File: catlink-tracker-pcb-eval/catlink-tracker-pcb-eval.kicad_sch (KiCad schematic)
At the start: 41 parts, among them J1 S2B-PH-K, J2 U.FL, J3 Header_01x03, J4 Header_02x02, J5 Header_02x03, J6 Header_01x02, J7 Header_01x06, J8 Header_01x05, SW1 SW_Push, U1 STM32L412K8Tx, U2 TLV75530PDBV, U3 Ai-Thinker-Ra-01S, U4 E108-GN03

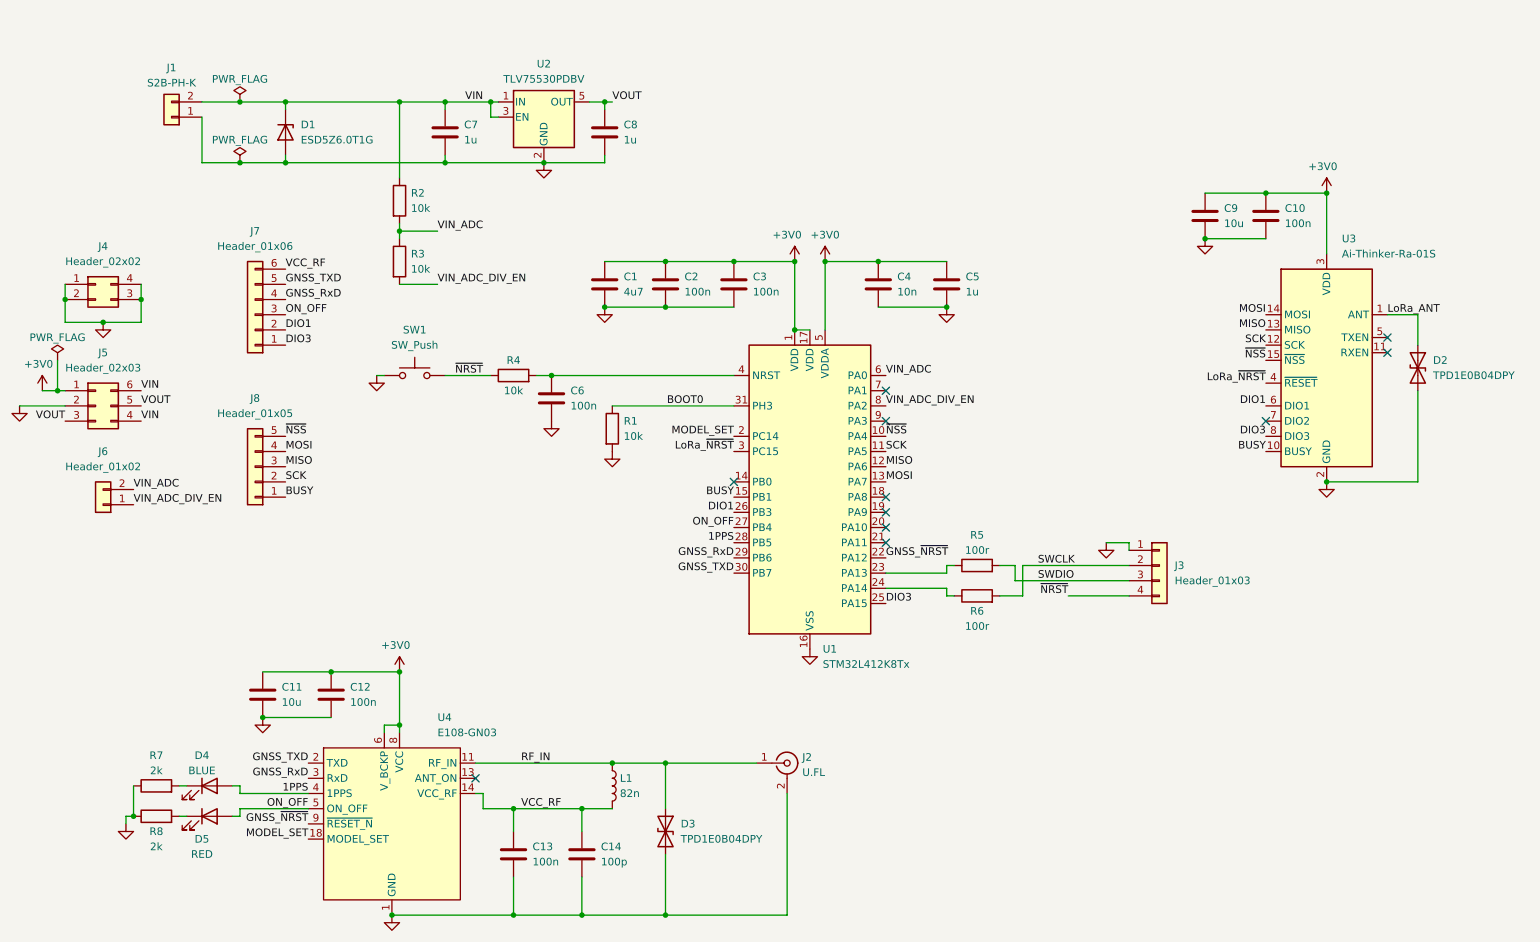
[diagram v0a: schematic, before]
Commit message: v0.1
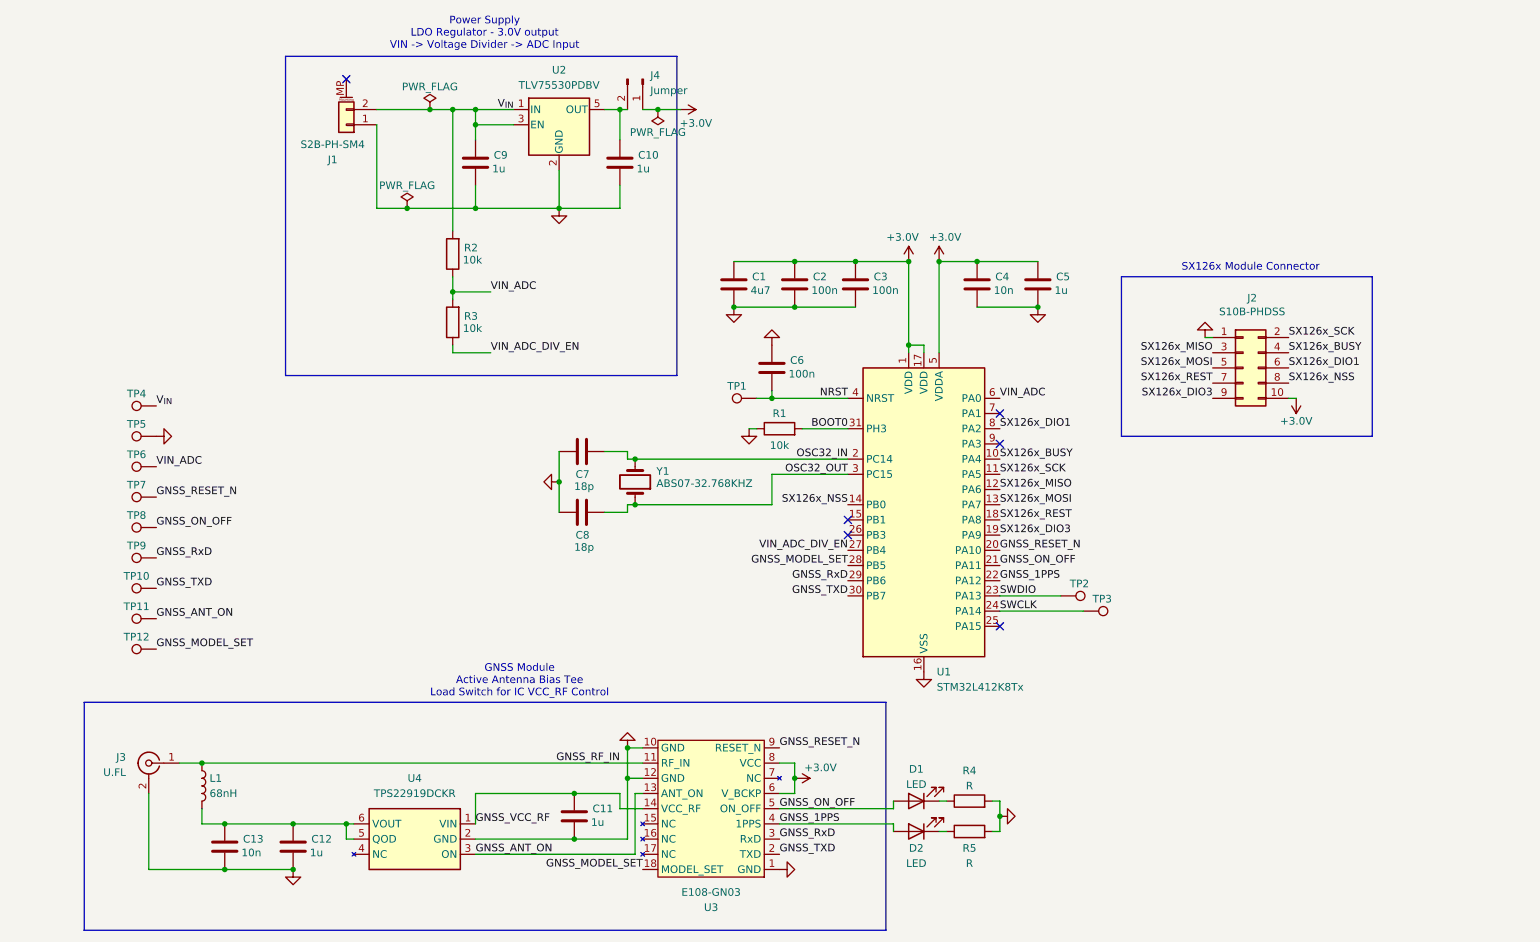
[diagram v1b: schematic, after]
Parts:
- removed C14: 100p, Custom:C_0603_1608Metric, symbol Device:C
- removed D1: ESD5Z6.0T1G, Custom:D_SOD-523, symbol Device:D_Zener
- removed D2, D3: TPD1E0B04DPY, Custom:D_Texas_DPY0002A_0.6x1mm_P0.65mm, symbol Device:D_TVS
- removed D4: BLUE, LED_THT:LED_D3.0mm, symbol Device:LED
- removed D5: RED, LED_THT:LED_D3.0mm, symbol Device:LED
- removed J1: S2B-PH-K, Connector_JST:JST_PH_S2B-PH-K_1x02_P2.00mm_Horizontal, symbol Connector_Generic:Conn_01x02
- removed J2: U.FL, Connector_Coaxial:U.FL_Hirose_U.FL-R-SMT-1_Vertical, symbol Connector:Conn_Coaxial
- removed J3: Header_01x03, Connector_PinHeader_2.54mm:PinHeader_1x04_P2.54mm_Vertical, symbol Connector_Generic:Conn_01x04
- removed J4: Header_02x02, Connector_PinHeader_2.54mm:PinHeader_2x02_P2.54mm_Vertical, symbol Connector_Generic:Conn_02x02_Counter_Clockwise
- removed J5: Header_02x03, Connector_PinHeader_2.54mm:PinHeader_2x03_P2.54mm_Vertical, symbol Connector_Generic:Conn_02x03_Counter_Clockwise
- removed J6: Header_01x02, Connector_PinHeader_2.54mm:PinHeader_1x02_P2.54mm_Vertical, symbol Connector_Generic:Conn_01x02
- removed J7: Header_01x06, Connector_PinHeader_2.54mm:PinHeader_1x06_P2.54mm_Vertical, symbol Connector_Generic:Conn_01x06
- removed J8: Header_01x05, Connector_PinHeader_2.54mm:PinHeader_1x05_P2.54mm_Vertical, symbol Connector_Generic:Conn_01x05
- removed R6: 100r, Custom:R_0603_1608Metric, symbol Device:R
- removed R7, R8: 2k, Resistor_THT:R_Axial_DIN0204_L3.6mm_D1.6mm_P1.90mm_Vertical, symbol Device:R
- removed SW1: SW_Push, Custom:SW_PUSH_5x7mm, symbol Switch:SW_Push
- removed U3: Ai-Thinker-Ra-01S, Custom:Ai-Thinker-Ra-01S, symbol Custom:Ai-Thinker-Ra-01S
- removed U4: E108-GN03, Custom:E108-GN03, symbol Custom:E108-GN03
- added D1, D2: LED, LED_THT:LED_D3.0mm, symbol Device:LED
- added J1: S2B-PH-SM4, Connector_JST:JST_PH_S2B-PH-SM4-TB_1x02-1MP_P2.00mm_Horizontal, symbol Connector_Generic_MountingPin:Conn_01x02_MountingPin
- added J2: S10B-PHDSS, Connector_JST:JST_PHD_S10B-PHDSS_2x05_P2.00mm_Horizontal, symbol Connector_Generic:Conn_02x05_Odd_Even
- added J3: U.FL, Connector_Coaxial:U.FL_Hirose_U.FL-R-SMT-1_Vertical, symbol Connector:Conn_Coaxial
- added J4: Jumper, Connector_PinHeader_2.54mm:PinHeader_1x02_P2.54mm_Vertical, symbol Connector:Conn_01x02_Pin
- added TP1, TP10, TP11, TP12, TP2, TP3, TP4, TP5, TP6, TP7, TP8, TP9: ~, Custom:TestPoint, symbol Connector:TestPoint
- added U3: E108-GN03, Custom:E108-GN03, symbol Custom:E108-GN03
- added U4: TPS22919DCKR, Package_TO_SOT_SMD:SOT-363_SC-70-6, symbol Custom:TPS22919DCKR
- added Y1: ABS07-32.768KHZ, Crystal:Crystal_SMD_3215-2Pin_3.2x1.5mm, symbol Device:Crystal
- C1, C2, C3, C4, C5, C6: footprint Custom:C_0603_1608Metric -> Capacitor_SMD:C_0603_1608Metric
- C10, C12: value 100n -> 1u; footprint Custom:C_0603_1608Metric -> Capacitor_SMD:C_0603_1608Metric
- C11, C9: value 10u -> 1u; footprint Custom:C_0805_2012Metric -> Capacitor_SMD:C_0603_1608Metric
- C13: value 100n -> 10n; footprint Custom:C_0603_1608Metric -> Capacitor_SMD:C_0603_1608Metric
- C7, C8: value 1u -> 18p; footprint Custom:C_0603_1608Metric -> Capacitor_SMD:C_0603_1608Metric
- L1: value 82n -> 68nH; footprint Custom:L_0603_1608Metric -> Inductor_SMD:L_0603_1608Metric
- R1, R2, R3: footprint Custom:R_0603_1608Metric -> Resistor_SMD:R_0603_1608Metric
- R4: value 10k -> R; footprint Custom:R_0603_1608Metric -> Resistor_THT:R_Axial_DIN0204_L3.6mm_D1.6mm_P1.90mm_Vertical
- R5: value 100r -> R; footprint Custom:R_0603_1608Metric -> Resistor_THT:R_Axial_DIN0204_L3.6mm_D1.6mm_P1.90mm_Vertical
- U1: footprint Custom:LQFP-32_7x7mm_P0.8mm -> Package_QFP:LQFP-32_7x7mm_P0.8mm
- U2: footprint Custom:SOT-23-5 -> Package_TO_SOT_SMD:SOT-23-5
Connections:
- net ON_OFF is gone; now on net VIN_ADC_DIV_EN: U1.27 (PB4)
- net BOOT0: now also R1.2; no longer R1.1
- net GND: now also C6.1, C7.1, C8.1, R1.1, R4.2, R5.2, J1.1 (Pin_1), J2.1 (Pin_1), J3.2 (Ext), TP5.1, U3.1 (GND), U3.10 (GND), U3.12 (GND), U4.2 (GND); no longer C6.2, C7.2, C8.2, R1.2
- net GNSS_RxD: now also TP9.1, U3.3 (RxD)
- net GNSS_TXD: now also TP10.1, U3.2 (TXD)
- net SWCLK: now also U1.24 (PA14), TP3.1
- net SWDIO: now also U1.23 (PA13), TP2.1; no longer R5.2
- net VIN_ADC: now also R2.1, R3.2, TP6.1; no longer R2.2, R3.1
- net VIN_ADC_DIV_EN: now also R3.1; no longer R3.2, U1.8 (PA2)
- net at R5.1: now also D2.1 (K); no longer U1.23 (PA13)
- net SX126x_NSS: now reaches U1.14 (PB0)
- net SX126x_NSS: now also J2.8 (Pin_8)
- net SX126x_REST: now reaches U1.18 (PA8)
- net SX126x_REST: now also J2.7 (Pin_7)
- net SX126x_DIO3: now reaches U1.19 (PA9)
- net SX126x_DIO3: now also J2.9 (Pin_9)
- net GNSS_RESET_N: now reaches U1.20 (PA10)
- net GNSS_RESET_N: now also TP7.1, U3.9 (RESET_N)
- net GNSS_ON_OFF: now reaches U1.21 (PA11)
- net GNSS_ON_OFF: now also D1.2 (A), TP8.1, U3.5 (ON_OFF)
- net +3V0 renamed +3.0V
- net +3.0V: now also J2.10 (Pin_10), J4.1 (Pin_1), U3.6 (V_BCKP), U3.8 (VCC); no longer C10.1, C11.1, C12.1, C9.1
- net 1PPS renamed GNSS_MODEL_SET
- net GNSS_MODEL_SET: now also TP12.1, U3.18 (MODEL_SET)
- net BUSY: no longer names the net of U1.15 (PB1)
- net DIO1: no longer names the net of U1.26 (PB3)
- net DIO3: no longer names the net of U1.25 (PA15)
- net GNSS_~{NRST} renamed GNSS_1PPS
- net GNSS_1PPS: now also D2.2 (A), U3.4 (1PPS)
- net LoRa_~{NRST} renamed OSC32_OUT
- net OSC32_OUT: now also C8.2, Y1.1
- net MISO renamed SX126x_MISO
- net SX126x_MISO: now also J2.3 (Pin_3)
- net MODEL_SET renamed OSC32_IN
- net OSC32_IN: now also C7.2, Y1.2
- net MOSI renamed SX126x_MOSI
- net SX126x_MOSI: now also J2.5 (Pin_5)
- net RF_IN renamed GNSS_RF_IN
- net GNSS_RF_IN: now also J3.1 (In), U3.11 (RF_IN)
- net SCK renamed SX126x_SCK
- net SX126x_SCK: now also J2.2 (Pin_2)
- net VCC_RF: no longer names the net of C13.1, L1.2
- net VCC_RF: now also C12.1, U4.5 (QOD), U4.6 (VOUT)
- net VIN renamed V_{IN}
- net V_{IN}: now also C9.1, R2.2, J1.2 (Pin_2), TP4.1; no longer C7.1, R2.1
- net VOUT: no longer names the net of U2.5 (OUT)
- net VOUT: now also C10.1, J4.2 (Pin_2); no longer C8.1
- net ~{NRST}: no longer names the net of R4.1
- net ~{NRST}: now also D1.1 (K)
- net ~{NSS} renamed SX126x_BUSY
- net SX126x_BUSY: now also J2.4 (Pin_4)
- new net GNSS_ANT_ON: TP11.1, U3.13 (ANT_ON), U4.3 (ON)
- new net GNSS_VCC_RF: C11.1, U3.14 (VCC_RF), U4.1 (VIN)
- new net NRST: C6.2, TP1.1, U1.4 (NRST)
- new net SX126x_DIO1: J2.6 (Pin_6), U1.8 (PA2)
- no-connect marks 11 -> 6
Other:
- note added: "GNSS Module Active Antenna Bias Tee Load Switch for IC VCC_RF Control"
- note added: "Power Supply LDO Regulator - 3.0V output VIN -> Voltage Divider -> ADC Input"
- note added: "SX126x Module Connector"
- title: CatLink Tracker Eval -> CatLink Development
